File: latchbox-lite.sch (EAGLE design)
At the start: 28 parts, among them IC1 PIC12F1822SO08

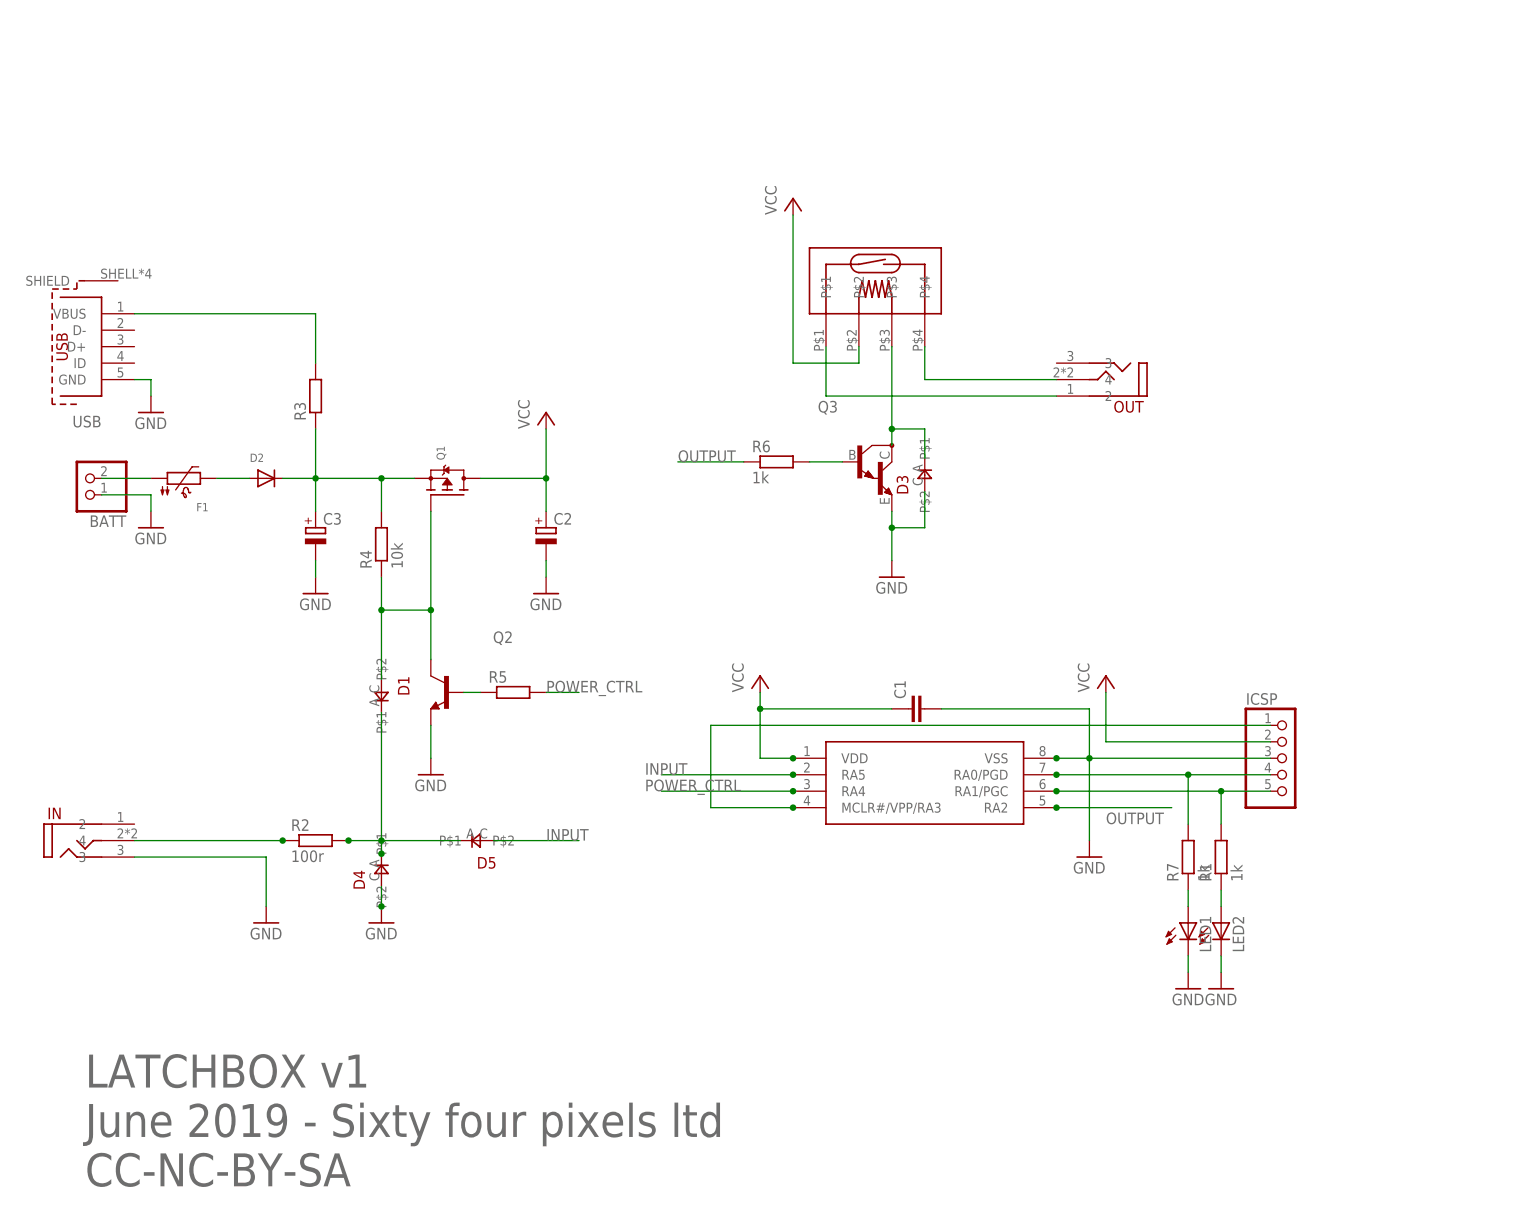
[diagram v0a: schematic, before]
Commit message: v2 possible
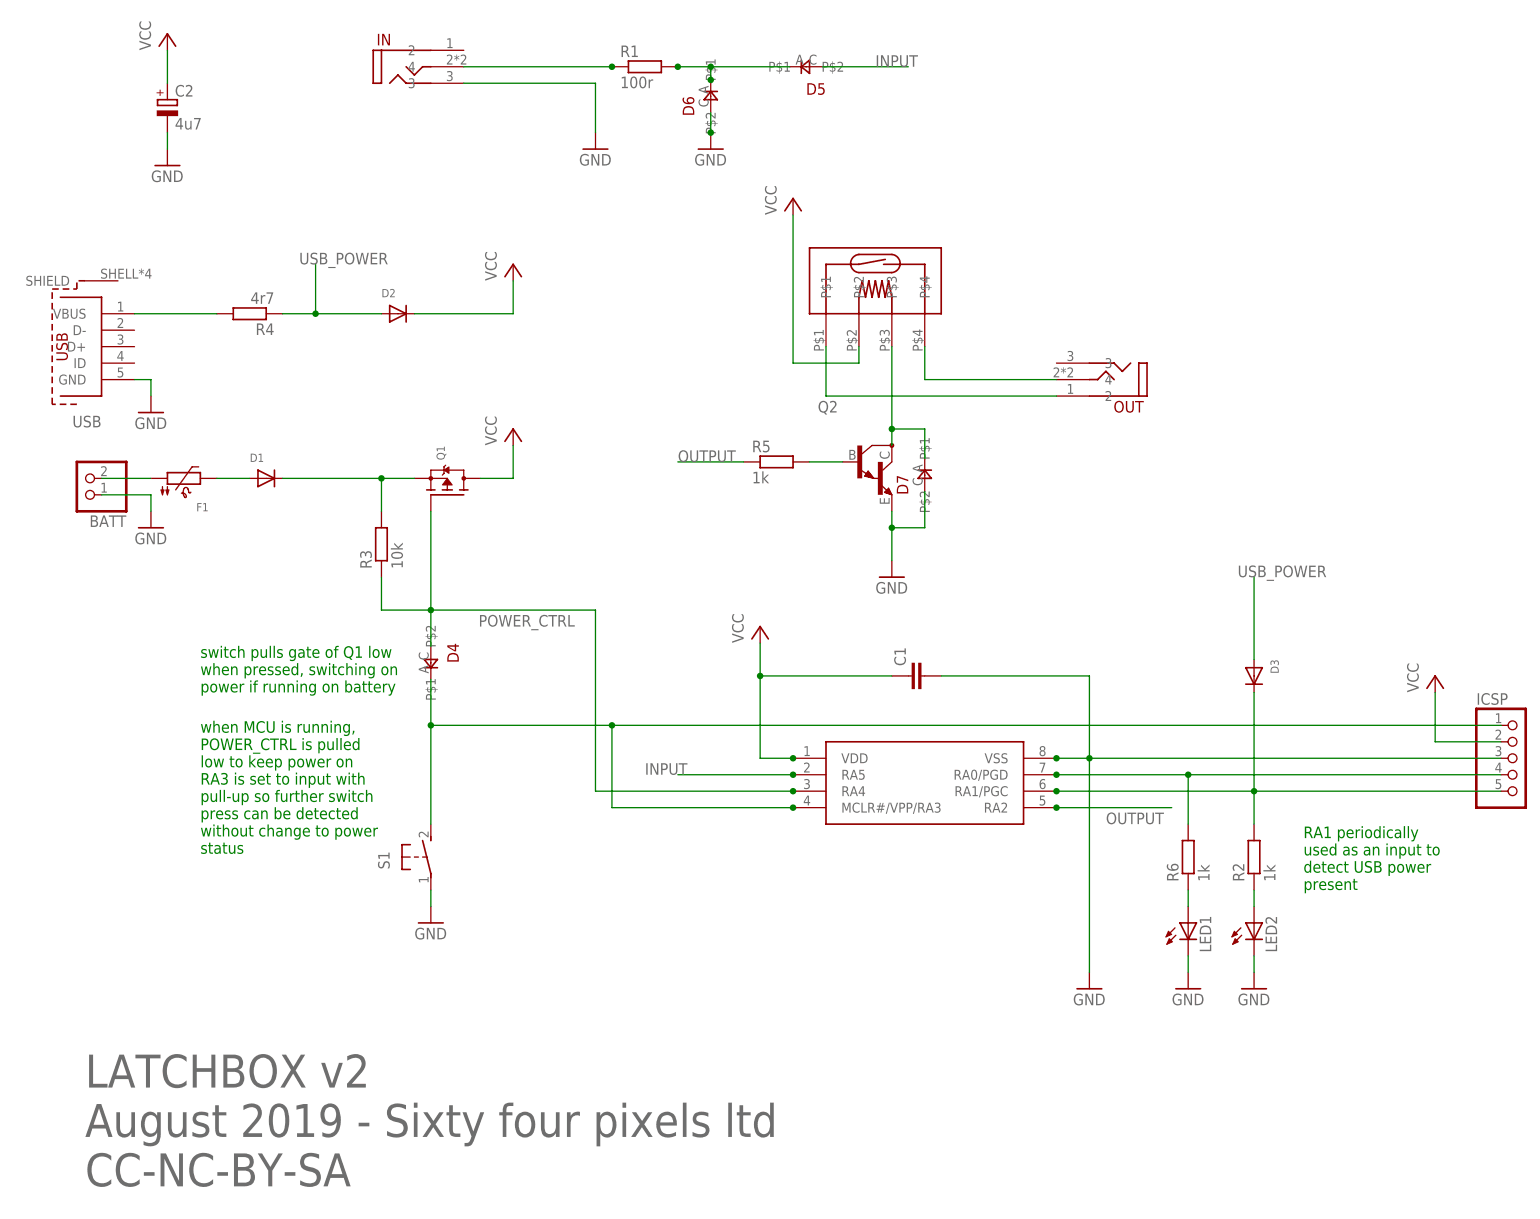
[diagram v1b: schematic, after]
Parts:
- removed C3: (no value), rcl:CPOL-EUE2,5-6E
- removed Q3: (no value), transistor:MMBTA13LT1-NPN_DARL-SOT23-BEC
- removed R7: 1k, rcl:R-EU_R0805
- added D6, D7: 0805DIODE, jasons_stuff:0805DIODE
- added S1: (no value), switch-omron:31-XX
- C2: value (none) -> 4u7
- D1, D3: value 0805DIODE -> (none); device jasons_stuff:0805DIODE -> microbuilder:DIODESOD-123
- Q2: device transistor:MMBT3904LT1-NPN-SOT23-BEC -> transistor:MMBTA13LT1-NPN_DARL-SOT23-BEC
- R1: value 1k -> 100r
- R2: value 100r -> 1k
- R3: value (none) -> 10k
- R4: value 10k -> 4r7
- R5: value (none) -> 1k
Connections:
- removed net N: D1.P$1, Q1.G, Q2.C, R4.1
- removed net N$2: Q2.B, R5.1
- new net USB_POWER: D2.A, D3.A, R4.1
- net GND: now also D6.P$1, D7.P$1, S1.P; no longer C3.-, D3.P$1, D4.P$1, Q3.E
- net N$1: now also R1.1; no longer R2.1
- net N$10: now also R6.1; no longer R7.1
- net N$11: now also R6.2; no longer R7.2
- net N$12: now also D3.C, R2.2; no longer R1.2
- net N$14: now also D4.P$2, S1.S
- net N$15: now also D1.A; no longer D2.A
- net N$16: now also R4.2; no longer R3.2
- net N$3: now also R2.1; no longer R1.1
- net N$4: now also D1.C, R3.2; no longer C3.+, D2.C, R3.1, R4.2
- net N$6: now also Q2.B, R5.2; no longer Q3.B, R6.2
- net N$9: now also D7.P$2, Q2.C; no longer D3.P$2, Q3.C
- net OUTPUT: now also R5.1; no longer R6.1
- net POWER_CTRL: now also D4.P$1, Q1.G, R3.1; no longer R5.2
- net VCC: now also D2.C
- net Z: now also D6.P$2, R1.2; no longer D1.P$2, D4.P$2, R2.2
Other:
- note added: "August 2019 - Sixty four pixels ltd"
- note added: "LATCHBOX v2"
- note added: "RA1 periodically used as an input to detect USB power present"
- note added: "switch pulls gate of Q1 low when pressed, switching on power if running on battery"
- note added: "when MCU is running, POWER_CTRL is pulled low to keep power on RA3 is set to input with pull-up so further switch press can be detected without change to power status"
- note removed: "June 2019 - Sixty four pixels ltd"
- note removed: "LATCHBOX v1"
- moved on the sheet: C1, C2, D2, D4, D5, ICSP, IN, LED2, R1, R2, R3, R4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
